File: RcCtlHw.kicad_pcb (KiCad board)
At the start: 2 copper layers, 26.7 x 41.9 mm, 30 parts, among them J1 USB_B_Mini, J2 Program, J3 TFT_LCD, SW1 On/Off, U1 TP4056, U2 ESP-M2, U3 ADS1015, U4 Joystick

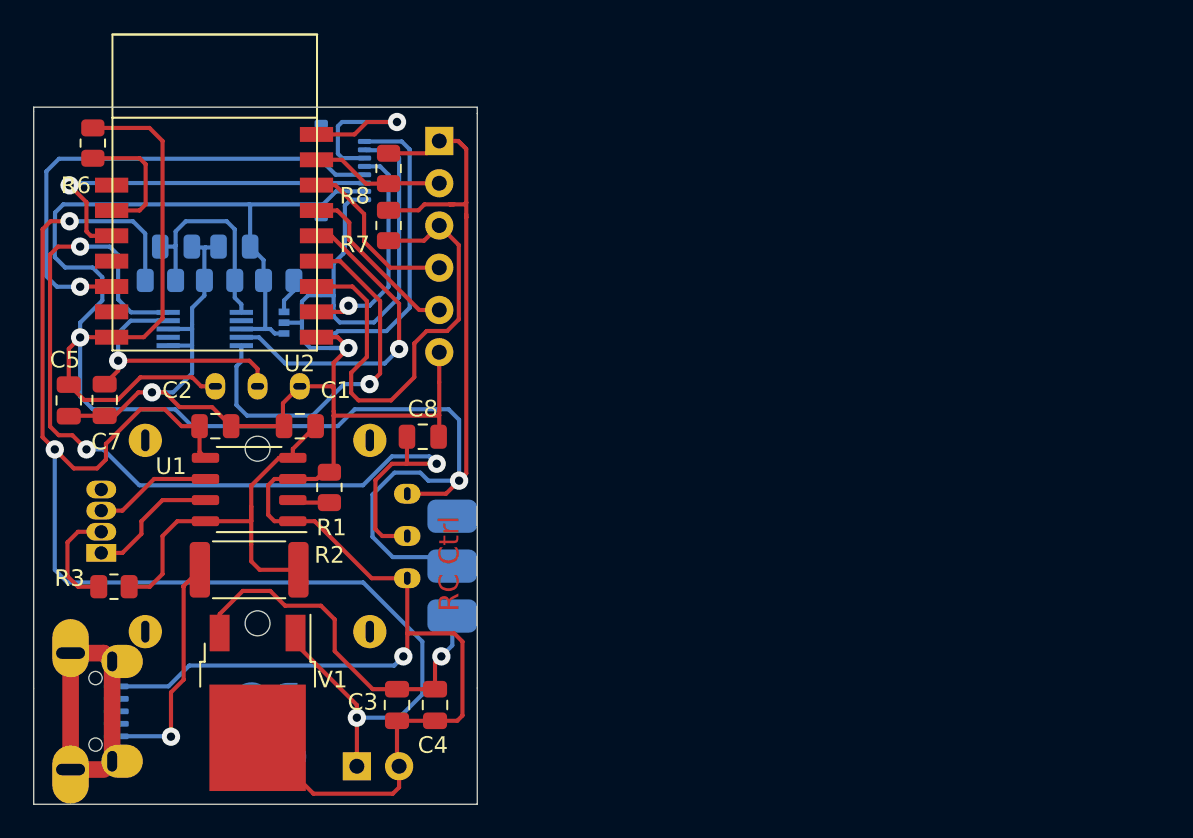
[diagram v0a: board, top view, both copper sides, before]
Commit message: Ready to etch
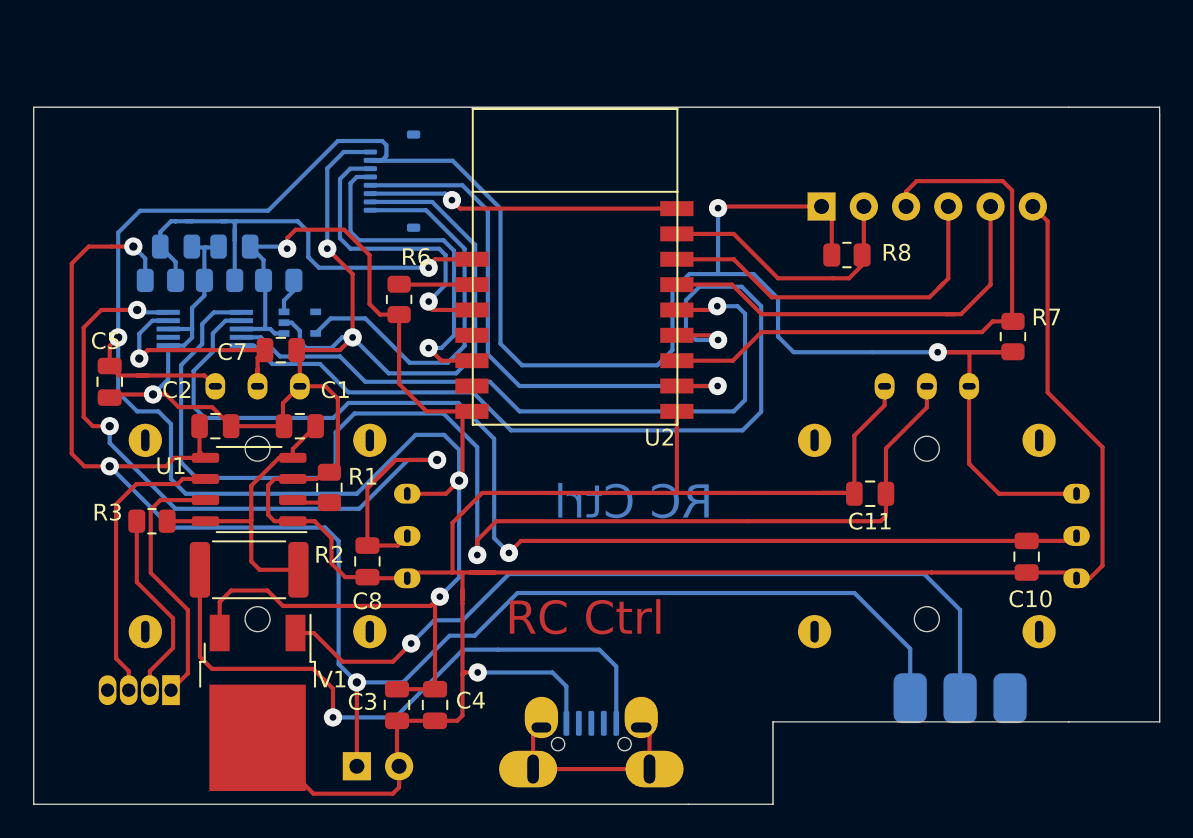
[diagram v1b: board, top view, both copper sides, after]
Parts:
- added C10: 100n, Capacitor_SMD:C_0805_2012Metric, F.Cu at (174.0, 111.5)
- added C11: 100n, Capacitor_SMD:C_0805_2012Metric, F.Cu at (164.6, 107.7)
- added U5: Left Joystick, TrevM:Joystick, B.Cu at (160.0, 110.2)
- D1: value LED_RCGB -> Chg
- R10: value 10K -> 1K
- U4: value Joystick -> Right Joystick
- V1: value Regulator -> 3V3
- moved R7 38.1 mm to (173.2, 98.2), turned to 90 degrees
- moved J1 36.4 mm to (147.8, 128.5), turned to 180 degrees
- moved R8 28.0 mm to (163.2, 93.3), turned to 0 degrees
- moved J2 23.3 mm to (161.7, 90.4), turned to 270 degrees
- moved U2 22.1 mm to (147.0, 98.0)
- moved R6 20.7 mm to (136.3, 96.0), turned to 90 degrees
- moved SW1 19.0 mm to (160.0, 121.5), turned to 90 degrees
- moved C7 11.0 mm to (129.2, 99.1), turned to 0 degrees
- moved D1 9.26 mm to (122.6, 119.5), turned to 180 degrees
- moved C8 8.20 mm to (134.4, 111.8), turned to 270 degrees
- moved J3 6.38 mm to (137.5, 88.9), turned to 270 degrees
- moved R3 4.55 mm to (121.4, 109.3)
- moved C5 2.71 mm to (118.9, 101.0)
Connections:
- net Net-(C7-Pad1) renamed /RH
- net Net-(C8-Pad1) renamed /RV
- C3 pad 1: Net-(C3-Pad1) -> +3V3
- C4 pad 1: Net-(C3-Pad1) -> +3V3
- SW1 pad 1: Net-(C3-Pad1) -> +BATT
- SW1 pad 2: +3V3 -> Net-(SW1-Pad2)
- U2 pad 1: (no net) -> Net-(C9-Pad1)
- U3 pad 6: Net-(C9-Pad1) -> /LH
- U3 pad 7: (no net) -> /LV
- V1 pad 1: +BATT -> Net-(SW1-Pad2)
- V1 pad 3: Net-(C3-Pad1) -> +3V3
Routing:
- net GND: track 154.4 -> 244.7 mm, vias 3 -> 4
- net /LH: track 0.00 -> 74.6 mm, vias 0 -> 1
- net +3V3: track 154.5 -> 225.0 mm, vias 2 -> 6
- net /LV: track 0.00 -> 68.3 mm, vias 0 -> 1
- net Net-(SW1-Pad2): track 0.00 -> 49.1 mm, vias 0 -> 1
- net /I2C_SCL: track 22.8 -> 52.1 mm
- net Net-(J1-Pad1): track 14.1 -> 38.3 mm
- net Net-(C3-Pad1): track 23.1 -> 0.00 mm, vias 1 -> 0
- net /I2C_SDA: track 19.9 -> 42.0 mm
- net /TFT_RS: track 13.3 -> 33.4 mm
- net Net-(C9-Pad1): track 13.1 -> 29.0 mm, vias 0 -> 1
- net /RX: track 10.5 -> 25.6 mm
- net +BATT: track 85.2 -> 98.1 mm
- net /TX: track 10.4 -> 22.4 mm
- net Net-(D1-Pad3): track 7.05 -> 17.5 mm
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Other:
- board size 26.7 x 41.9 mm -> 67.7 x 41.9 mm
- board text removed: "Ctrl"
- board text removed: "RC"
